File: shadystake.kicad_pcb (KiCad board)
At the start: 2 copper layers, 96.8 x 181.5 mm, 28 parts, among them J1 6P6C, J2 6P6C, J3 6P6C, J4 6P6C, J5 6P6C, J6 6P6C, J7 8P8C

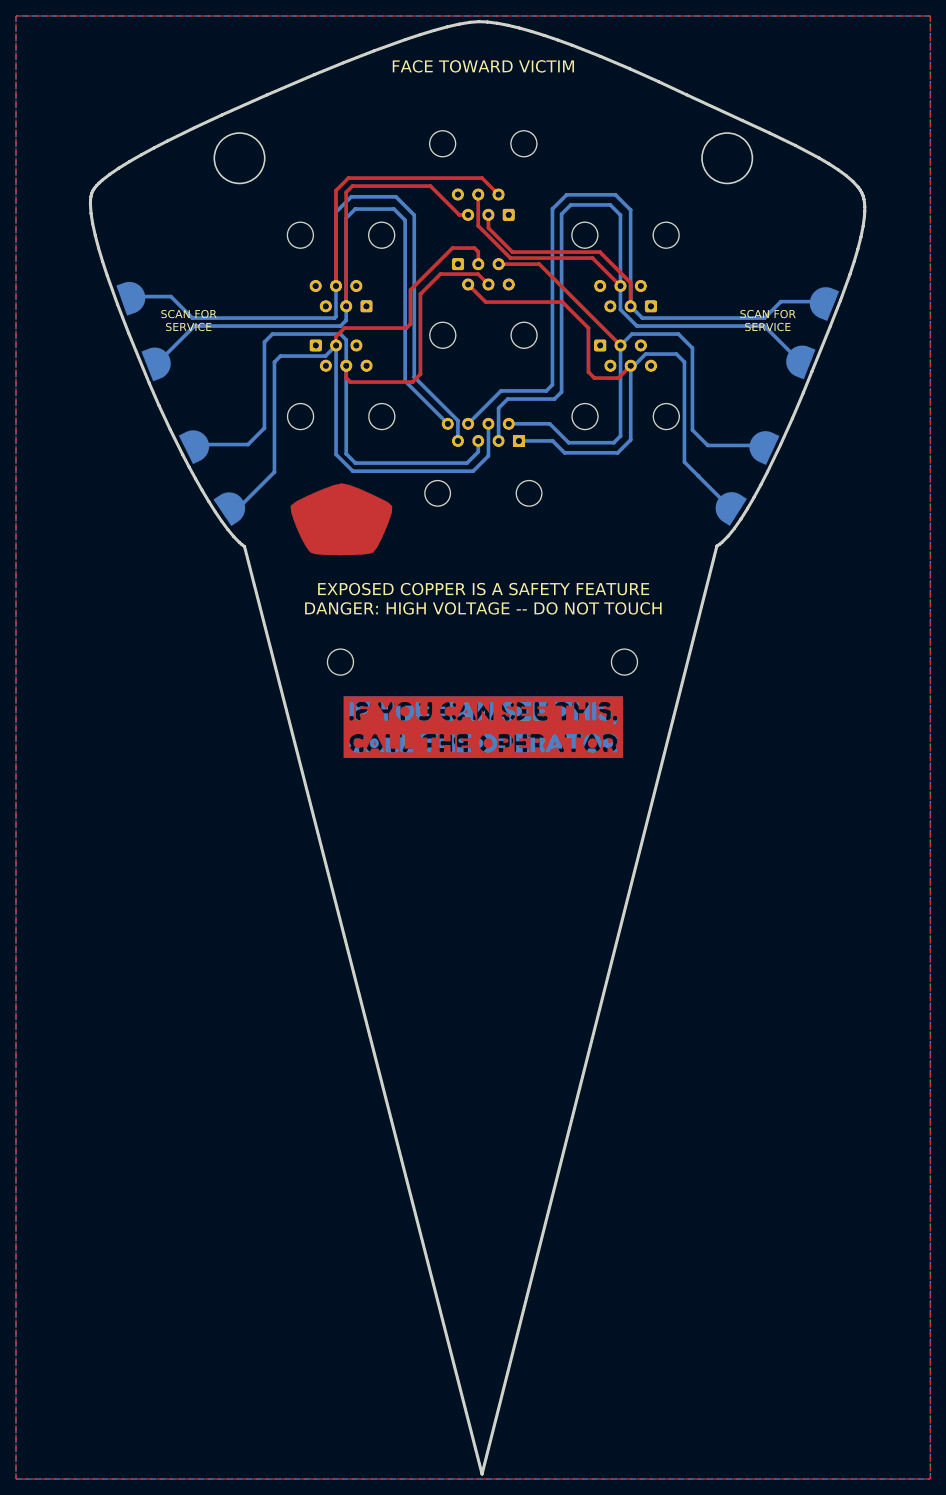
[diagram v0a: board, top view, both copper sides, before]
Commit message: Reimport edge.cuts... jfc...
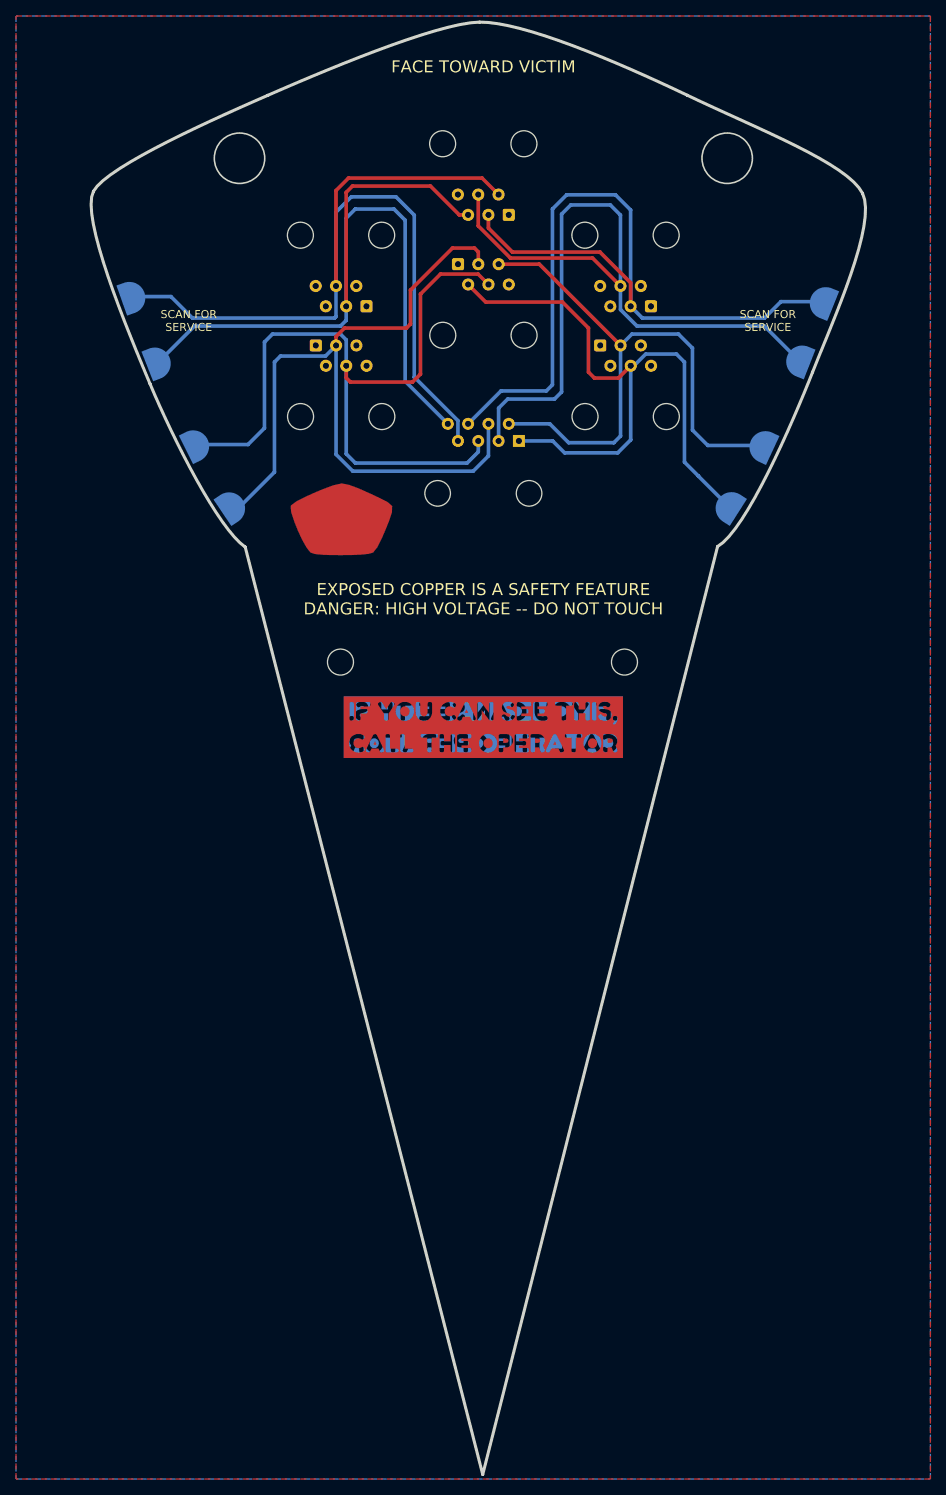
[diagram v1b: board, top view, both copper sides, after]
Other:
- outline, holes or cut-outs redrawn
